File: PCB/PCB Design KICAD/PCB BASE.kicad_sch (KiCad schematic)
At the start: 0 parts

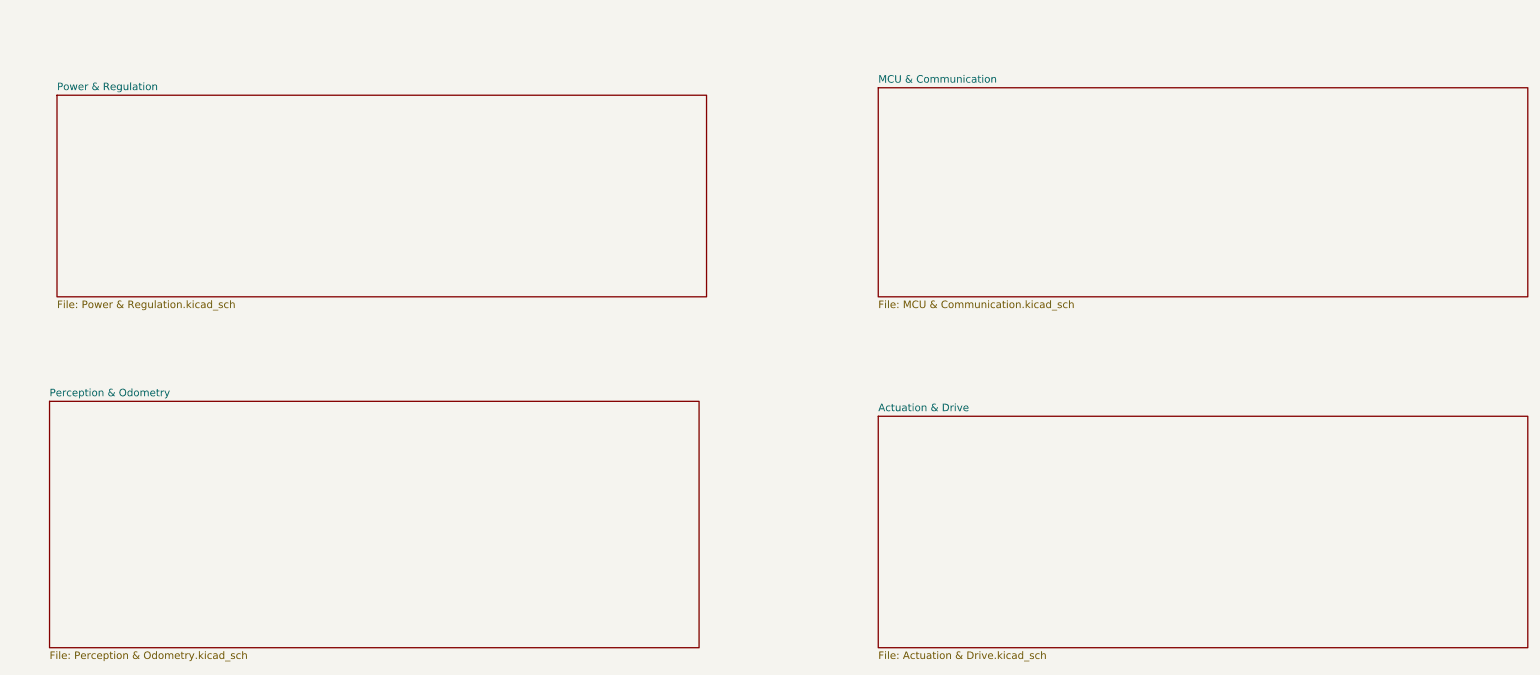
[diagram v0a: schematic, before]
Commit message: FINAL SCHEMATIC
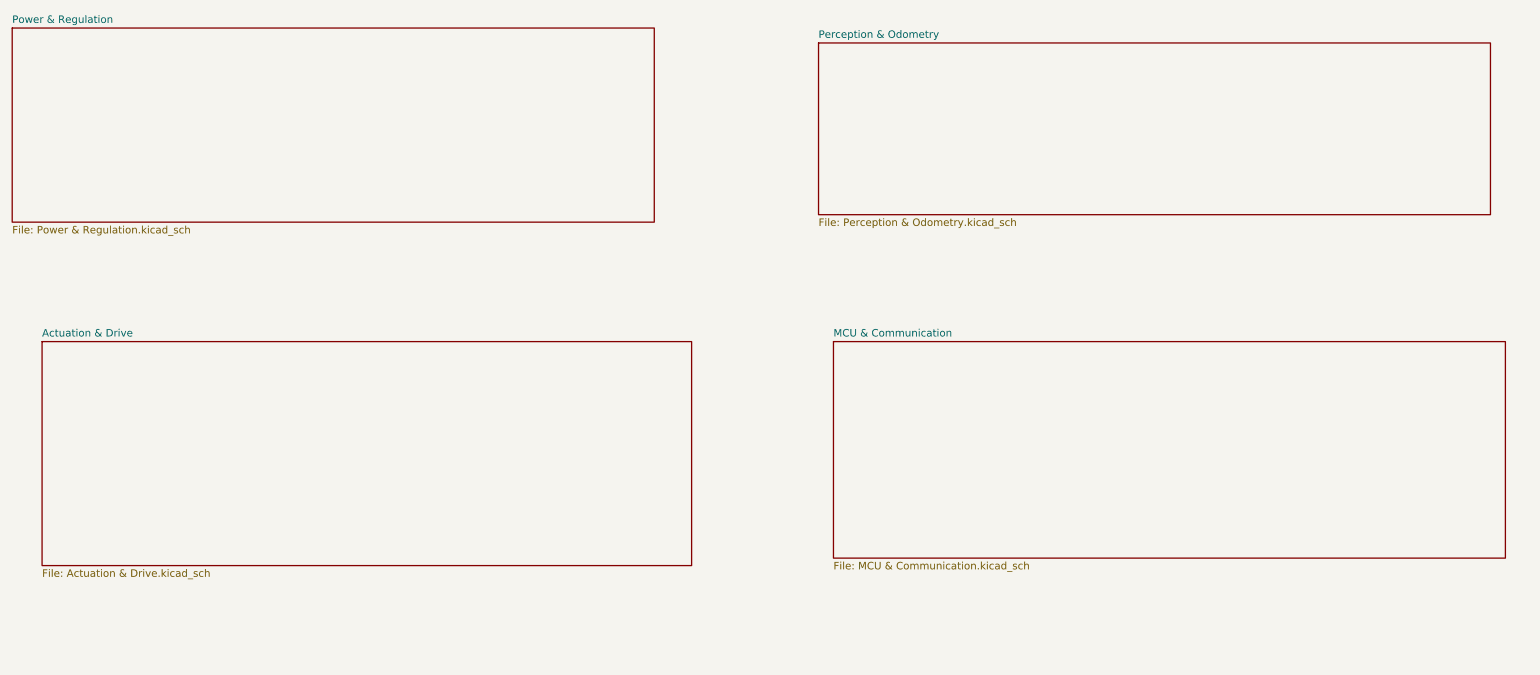
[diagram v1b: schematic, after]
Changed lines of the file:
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@@
 	(paper "A4")
 	(sheet
-		(at 24.13 27.94)
-		(size 110.49 34.29)
+		(at 21.59 69.85)
+		(size 110.49 38.1)
+		(exclude_from_sim no)
+		(in_bom yes)
+		(on_board yes)
+		(dnp no)
+		(fields_autoplaced yes)
+		(stroke
+			(width 0.1524)
+			(type solid)
+		)
+		(fill
+			(color 0 0 0 0.0000)
+		)
+		(property "Sheetname" "Actuation & Drive"
+			(at 21.59 69.1384 0)
+			(effects
+				(font
+					(size 1.27 1.27)
+				)
+				(justify left bottom)
+			)
+		)
+		(property "Sheetfile" "Actuation & Drive.kicad_sch"
+			(at 21.59 108.5346 0)
+			(effects
+				(font
+					(size 1.27 1.27)
+				)
+				(justify left top)
+			)
+		)
+		(instances
+			(project "PCB BASE"
+				(path "/8e4f15b9-abd6-436a-9fb0-d895efa0c8c7"
+					(page "4")
+				)
+			)
+		)
+	)
+	(sheet
+		(at 153.67 19.05)
+		(size 114.3 29.21)
+		(exclude_from_sim no)
+		(in_bom yes)
+		(on_board yes)
+		(dnp no)
+		(fields_autoplaced yes)
+		(stroke
+			(width 0.1524)
+			(type solid)
+		)
+		(fill
+			(color 0 0 0 0.0000)
+		)
+		(property "Sheetname" "Perception & Odometry"
+			(at 153.67 18.3384 0)
+			(effects
+				(font
+					(size 1.27 1.27)
+				)
+				(justify left bottom)
+			)
+		)
+		(property "Sheetfile" "Perception & Odometry.kicad_sch"
+			(at 153.67 48.8446 0)
+			(effects
+				(font
+					(size 1.27 1.27)
+				)
+				(justify left top)
+			)
+		)
+		(instances
+			(project "PCB BASE"
+				(path "/8e4f15b9-abd6-436a-9fb0-d895efa0c8c7"
+					(page "3")
+				)
+			)
+		)
+	)
+	(sheet
+		(at 16.51 16.51)
+		(size 109.22 33.02)
 		(exclude_from_sim no)
 		(in_bom yes)
@@
 		)
 		(property "Sheetname" "Power & Regulation"
-			(at 24.13 27.2284 0)
+			(at 16.51 15.7984 0)
 			(effects
 				(font
@@
 		)
 		(property "Sheetfile" "Power & Regulation.kicad_sch"
-			(at 24.13 62.8146 0)
+			(at 16.51 50.1146 0)
 			(effects
 				(font
@@
 		)
 		(instances
-			(project "Base Circuit"
-				(path "/45296ee7-52c3-4bc6-b17b-9e2c5f0e6ce0"
+			(project "PCB BASE"
+				(path "/8e4f15b9-abd6-436a-9fb0-d895efa0c8c7"
 					(page "2")
 				)
@@
 	)
 	(sheet
-		(at 163.83 82.55)
-		(size 110.49 39.37)
-		(exclude_from_sim no)
-		(in_bom yes)
-		(on_board yes)
-		(dnp no)
-		(fields_autoplaced yes)
-		(stroke
-			(width 0.1524)
-			(type solid)
-		)
-		(fill
-			(color 0 0 0 0.0000)
-		)
-		(property "Sheetname" "Actuation & Drive"
-			(at 163.83 81.8384 0)
-			(effects
-				(font
-					(size 1.27 1.27)
-				)
-				(justify left bottom)
-			)
-		)
-		(property "Sheetfile" "Actuation & Drive.kicad_sch"
-			(at 163.83 122.5046 0)
-			(effects
-				(font
-					(size 1.27 1.27)
-				)
-				(justify left top)
-			)
-		)
-		(instances
-			(project "Base Circuit"
-				(path "/45296ee7-52c3-4bc6-b17b-9e2c5f0e6ce0"
-					(page "4")
-				)
-			)
-		)
-	)
-	(sheet
-		(at 163.83 26.67)
-		(size 110.49 35.56)
+		(at 156.21 69.85)
+		(size 114.3 36.83)
 		(exclude_from_sim no)
 		(in_bom yes)
@@
 		)
 		(property "Sheetname" "MCU & Communication"
-			(at 163.83 25.9584 0)
+			(at 156.21 69.1384 0)
 			(effects
 				(font
@@
 		)
 		(property "Sheetfile" "MCU & Communication.kicad_sch"
-			(at 163.83 62.8146 0)
+			(at 156.21 107.2646 0)
 			(effects
 				(font
@@
 		)
 		(instances
-			(project "Base Circuit"
-				(path "/45296ee7-52c3-4bc6-b17b-9e2c5f0e6ce0"
-					(page "6")
+			(project "PCB BASE"
+				(path "/8e4f15b9-abd6-436a-9fb0-d895efa0c8c7"
+					(page "5")
 				)
 			)
-		)
-	)
-	(sheet
-		(at 22.86 80.01)
-		(size 110.49 41.91)
-		(exclude_from_sim no)
-		(in_bom yes)
-		(on_board yes)
-		(dnp no)
-		(fields_autoplaced yes)
-		(stroke
-			(width 0.1524)
-			(type solid)
-		)
-		(fill
-			(color 0 0 0 0.0000)
-		)
-		(property "Sheetname" "Perception & Odometry"
-			(at 22.86 79.2984 0)
-			(effects
-				(font
-					(size 1.27 1.27)
-				)
-				(justify left bottom)
-			)
-		)
-		(property "Sheetfile" "Perception & Odometry.kicad_sch"
-			(at 22.86 122.5046 0)
-			(effects
-				(font
-					(size 1.27 1.27)
-				)
-				(justify left top)
-			)
-		)
-		(instances
-			(project "Base Circuit"
-				(path "/45296ee7-52c3-4bc6-b17b-9e2c5f0e6ce0"
-					(page "4")
-				)
-			)
